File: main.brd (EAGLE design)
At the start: 130 x 34 mm, 176 parts, among them CN1 DC-012A-D010, CN2 JST GH 6P V-TH, CN3 5.8ZSPT, CN4 8 PIN FFC, CN5 MC-118LS-H100, CN6 JST GH 6P V-TH, CN7 8 PIN FFC, Q1 GSFP0449, Q6 IRLML6244, U1 Ti60F225C4, U10 W958D8NBYA5I, U11 TPS70918, U12 AP7335, U2 USBLC6-2SC6, U24 SCHMITT, U25 SCHMITT, U3 93LC56B-I/SN, U4 W25Q128JV, U5 TPS62065, U6 FT2232H, U7 TPS563201, U8 AR0822, U9 TPS62065

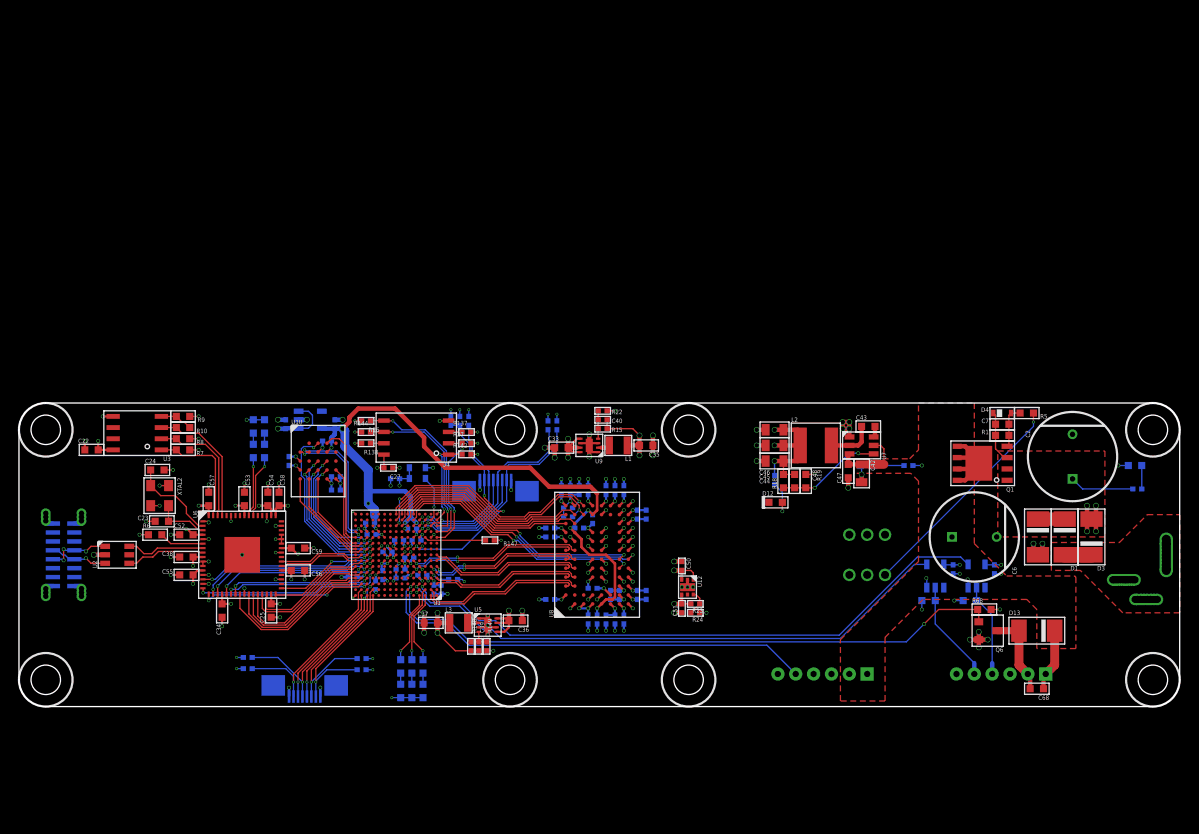
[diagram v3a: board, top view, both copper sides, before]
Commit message: Moving back to Trion
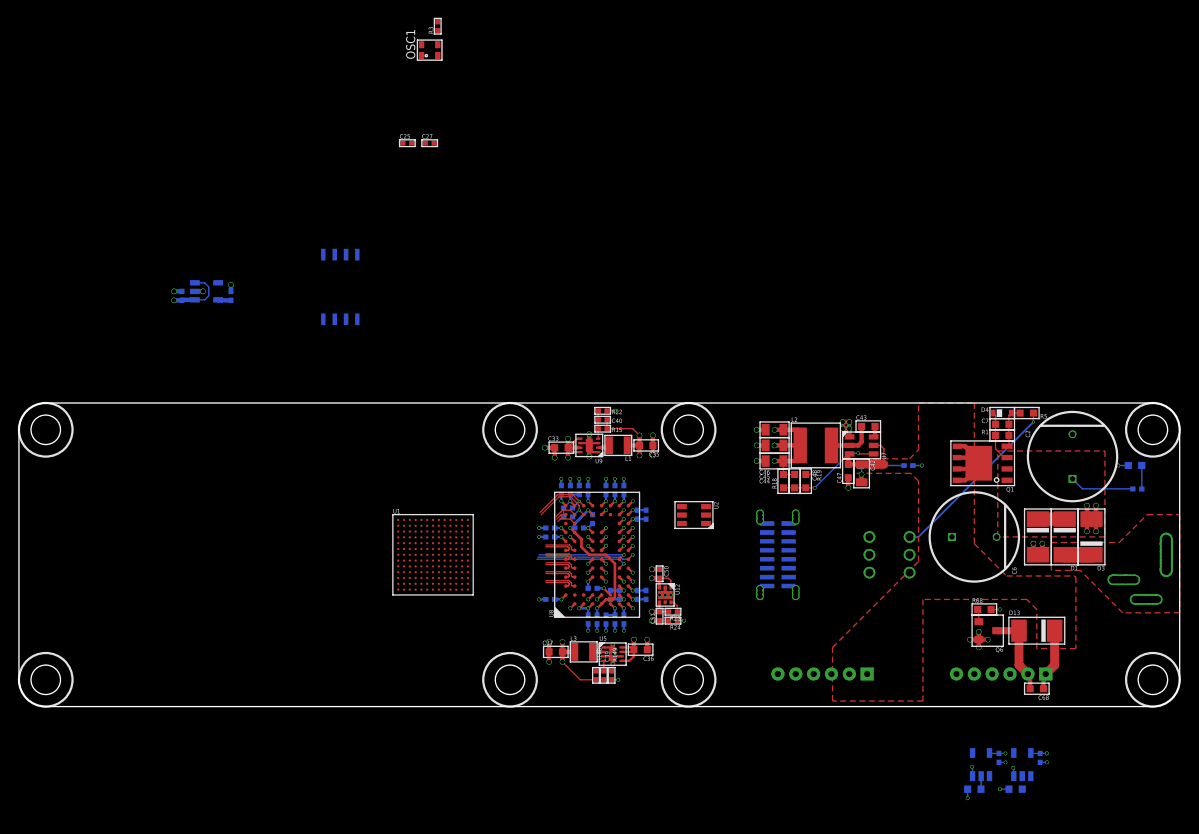
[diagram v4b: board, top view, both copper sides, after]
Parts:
- removed C22, C34, C38, C52, C53, C54, C55, C56, C57, C59: 0.1uF 16V, c_0603:0603
- removed C23, C24: 10pF 100V, c_0603:0603
- removed C28, C61, C62, C63, C64, C66, C67, C71, C72, C73, C74, C75, C77, C78, C79, C80, C81, C82: 0.1uF 16V, c_0402:0402
- removed C58: 4.7uF 6.3V, c_0603:0603
- removed C65, C76, C83: 10uF 6.3V, c_0402:0402
- removed CN4, CN7: 8 PIN FFC, CONNECTORs:SFV8R-1STBE1HLF
- removed D10, D12, D5, D6, D7, D8: RED LED, OPTO:0603_POLAR
- removed R10, R11, R12, R13, R14, R59: 2.2k, r_0603:0603
- removed R130, R137, R138, R142, R143, R144, R145, R146, R147, R20, R21, R26, R27, R74, R75: 10k, r_0402:0402
- removed R6: 12k, RESISTORS:0603
- removed R67: 1k, r_0402:0402
- removed R7, R8, R9: 10k, r_0603:0603
- removed U10: W958D8NBYA5I, ICs:VBGA24
- removed U3: 93LC56B-I/SN, ICs:SO8
- removed U4: W25Q128JV, ICs:SO8-208MIL
- removed U6: FT2232H, ICs:QFN64
- removed XTAL2: 12MHz, CRYSTALS:3.2X3.5SMD
- added U37: W25Q128JV, ICs:SO8-208MIL
- C25: value 0.1uF 16V -> 0.1uF 10V; device c_0603:0603 -> c_0402:0402
- C27: value 0.1uF 16V -> 0.1uF 10V
- R3: value 10k -> 10R
- U1: value Ti60F225C4 -> T20F169; device ICs:FBGA225 -> ICs:FBGA169
- moved CN5 80.0 mm to (20.0, 0.00), turned to 270 degrees
- moved U2 64.8 mm to (10.6, 4.45), turned to 270 degrees
- moved C25 54.5 mm to (-21.5, 46.1), turned to 0 degrees
- moved OSC1 47.4 mm to (-19.0, 56.5), flipped to the top, turned to 0 degrees
- moved R3 46.4 mm to (-18.1, 59.2), flipped to the top
- moved C27 36.6 mm to (-19.0, 46.1), turned to 0 degrees
- moved C69 21.7 mm to (49.4, -22.8)
- moved C70 21.7 mm to (44.8, -22.8)
- moved R72 21.7 mm to (46.6, -26.2)
- moved R73 21.7 mm to (42.0, -26.2)
- moved U24 21.7 mm to (47.4, -23.5)
- moved U25 21.7 mm to (42.8, -23.5)
- moved C41 18.5 mm to (-46.8, 29.0)
- moved C49 18.5 mm to (-41.2, 29.0)
- moved U11 18.5 mm to (-44.0, 29.5)
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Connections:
- removed net FLS_NHOLD: R138.1, U4.7
- removed net FLS_SPI_CLK: R144.1, U1.N1, U4.6
- removed net FLS_SPI_MISO: R27.1, U1.L1, U4.2
- removed net FLS_SPI_MOSI: R26.1, U1.M1, U4.5
- removed net FLS_SPI_NCS: R142.1, U1.P1, U4.1
- removed net FPGA_CLK_33M: OSC1.3, U1.P2
- removed net FPGA_CONF_CDONE: R147.1, U1.L3
- removed net FPGA_CONF_CSI: CN4.3, R145.1, U1.N2
- removed net FPGA_CONF_NCRST: C66.2, CN4.2, R146.1, U1.J5
- removed net FPGA_CONF_NTEST: R143.1, U1.E2
- removed net FPGA_JTAG_TCK: CN4.5, R3.1, U1.N4
- removed net FPGA_JTAG_TDI: CN4.4, U1.P3
- removed net FPGA_JTAG_TDO: CN4.7, R130.1, U1.M4
- removed net FPGA_JTAG_TMS: CN4.6, U1.N3
- removed net FT_CLKOUT: U1.G14, U6.32
- removed net FT_CONT_RX: U1.H14, U6.39
- removed net FT_CONT_TX: U1.G15, U6.38
- removed net FT_D0: U1.C13, U6.16
- removed net FT_D1: U1.C14, U6.17
- removed net FT_D2: U1.G13, U6.18
- removed net FT_D3: U1.F13, U6.19
- removed net FT_D4: U1.F12, U6.21
- removed net FT_D5: U1.E12, U6.22
- removed net FT_D6: U1.D13, U6.23
- removed net FT_D7: U1.C15, U6.24
- removed net FT_NOE: U1.H13, U6.33
- removed net FT_NRD: U1.E14, U6.28
- removed net FT_NRST: U1.H12, U6.14
- removed net FT_NRXF: U1.D14, U6.26
- removed net FT_NSIWU: U1.F15, U6.30
- removed net FT_NTXE: U1.D15, U6.27
- removed net FT_NWR: U1.E15, U6.29
- removed net LED_FPGA_STATUS: D6.K, U1.A4
- removed net LED_FT_CONT_NRXLED: D8.K, U6.54
- removed net LED_FT_CONT_NTXLED: D7.K, U6.55
- removed net LED_PROC_SCANNING: D10.K, U1.A3
- removed net LED_PROC_STATUS: D5.K, U1.B3
- removed net LED_USB_ACT: D12.K
- removed net N$113: D10.A, R59.1
- removed net N$14: D5.A, R11.1
- removed net N$15: D6.A, R12.1
- removed net N$16: D7.A, R13.1
- removed net N$17: D8.A, R14.1
- removed net N$42: R6.2, U6.6
- removed net N$43: R7.1, U3.1, U6.63
- removed net N$44: R8.1, U3.2, U6.62
- removed net N$45: R10.2, U3.3, U6.61
- removed net N$46: R10.1, R9.1, U3.4
- removed net N$47: D12.A, R67.1
- removed net N$49: C23.2, U6.3, XTAL2.3
- removed net N$50: C24.2, U6.2, XTAL2.1
- removed net N$51: C55.2, C56.2, C57.2, C58.2, U6.12, U6.37, U6.49, U6.64
- removed net N$8: R137.1, U4.3
- removed net PROC_JTAG_TCK: CN7.5, R21.1, U1.C12
- removed net PROC_JTAG_TDI: CN7.4, U1.A13
- removed net PROC_JTAG_TDO: CN7.7, R20.1, U1.B14
- removed net PROC_JTAG_TMS: CN7.6, U1.A14
- removed net PROC_UART_RX: CN7.2, R75.1, U1.A12
- removed net PROC_UART_TX: CN7.3, R74.1, U1.B12
- removed net PWR_MIPI_1V2: C75.2, C76.2, R143.2, U1.D2, U1.F4
- removed net RAM_CLKN: U1.M15, U10.B1
- removed net RAM_CLKP: U1.M14, U10.B2
- removed net RAM_D0: U1.K13, U10.D3
- removed net RAM_D1: U1.J13, U10.D2
- removed net RAM_D2: U1.L12, U10.C4
- removed net RAM_D3: U1.L13, U10.D4
- removed net RAM_D4: U1.K15, U10.D5
- removed net RAM_D5: U1.K14, U10.E3
- removed net RAM_D6: U1.J15, U10.E2
- removed net RAM_D7: U1.J14, U10.E1
- removed net RAM_NCS: U1.J12, U10.A3
- removed net RAM_NRESET: U1.L15, U10.A4
- removed net RAM_RWDS: U1.K12, U10.C3
- new net N$9: OSC1.3, R3.1
- new net PSS_CLK_33M: R3.2
- new net PSS_FLASH_D0: U37.5
- new net PSS_FLASH_D1: U37.2
- new net PSS_FLASH_D2: U37.3
- new net PSS_FLASH_D3: U37.7
- new net PSS_FLASH_NCS: U37.1
- new net PSS_FLASH_SCLK: U37.6
- new net USB_VBUS: CN5.A4, CN5.A9, CN5.B4, CN5.B9, U2.5
- net AR_CLK: no longer U1.P6
- net AR_GPIO0: no longer U1.P7
- net AR_GPIO1: no longer U1.R6
- net AR_GPIO2: no longer U1.P8
- net AR_GPIO3: no longer U1.R7
- net AR_I2C_SCL: no longer U1.R8
- net AR_I2C_SDA: no longer U1.N8
- net AR_MIPI_CLK_N: no longer U1.G1
- net AR_MIPI_CLK_P: no longer U1.H1
- net AR_MIPI_D0_N: no longer U1.F5
- net AR_MIPI_D0_P: no longer U1.G5
- net AR_MIPI_D1_N: no longer U1.F2
- net AR_MIPI_D1_P: no longer U1.F1
- net AR_MIPI_D2_N: no longer U1.C1
- net AR_MIPI_D2_P: no longer U1.D1
- net AR_MIPI_D3_N: no longer U1.A2
- net AR_MIPI_D3_P: no longer U1.B2
- net AR_NRESET: no longer U1.R5
- net AR_XSHUTDOWN: no longer U1.P5
- net GND: now also U37.4; no longer C22.1, C23.1, C24.1, C28.2, C34.1, C38.1, C52.1, C53.1, C54.1, C55.1, C56.1, C57.1, C58.1, C59.1, C61.1, C62.1, C63.1, C64.1, C65.1, C66.1, C67.1, C71.1, C72.1, C73.1, C74.1, C75.1, C76.1, C77.1, C78.1, C79.1, C80.1, C81.1, C82.1, C83.1, CN4.8, CN7.8, R6.1, U1.A1, U1.A15, U1.D3, U1.G6, U1.G8, U1.H7, U1.H9, U1.J6, U1.J8, U1.M13, U1.R1, U1.R15, U10.B3, U10.C1, U10.E5, U3.5, U4.4, U6.1, U6.10, U6.11, U6.13, U6.15, U6.25, U6.35, U6.41, U6.43, U6.44, U6.45, U6.47, U6.5, U6.51, U6.PAD, XTAL2.2, XTAL2.4
- net LED_PWM_CONT: no longer U1.C5
- net MTR_CONT_PWM: no longer U1.B5
- net MTR_SENSE_A: no longer U1.C3
- net MTR_SENSE_B: no longer U1.C4
- net PWR_FPGA_0V95: no longer C61.2, C62.2, C63.2, C64.2, C65.2, C67.2, C71.2, C72.2, C73.2, U1.E13, U1.E5, U1.G10, U1.G7, U1.G9, U1.H6, U1.H8, U1.J7, U1.J9, U1.L10, U1.L5, U1.M3
- net PWR_SYS_1V8: now also C25.2, OSC1.1, OSC1.4; no longer C74.2, C77.2, C78.2, C79.2, C80.2, C81.2, C82.2, C83.2, U1.D4, U1.E11, U1.J11, U1.L14, U1.L4, U1.M11, U1.N5, U1.N7, U10.B4, U10.D1, U10.E4
- net PWR_SYS_3V3: now also U37.8; no longer C22.2, C25.2, C28.1, C34.2, C38.2, C52.2, C53.2, C54.2, C59.2, CN4.1, CN7.1, OSC1.1, OSC1.4, R11.2, R12.2, R13.2, R130.2, R137.2, R138.2, R14.2, R142.2, R144.2, R145.2, R146.2, R147.2, R20.2, R21.2, R26.2, R27.2, R3.2, R59.2, R67.2, R7.2, R74.2, R75.2, R8.2, R9.2, U1.B13, U1.B4, U1.F14, U1.G12, U1.J4, U1.L2, U1.P4, U3.8, U4.8, U6.20, U6.31, U6.4, U6.42, U6.50, U6.56, U6.59, U6.9
- net USB_D_N: no longer U6.7
- net USB_D_P: no longer U6.8
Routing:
- net PWR_SYS_1V8: track 126.2 -> 27.1 mm, vias 17 -> 4
- net MTR_CONT_PWM: track 70.6 -> 1.43 mm, vias 2 -> 0
- net MTR_SENSE_A: track 68.3 -> 0.00 mm, vias 1 -> 0
- net MTR_SENSE_B: track 63.9 -> 0.00 mm, vias 1 -> 0
- net GND: track 161.7 -> 100.7 mm, vias 156 -> 97
- net PWR_SYS_3V3: track 95.1 -> 43.9 mm, vias 50 -> 10
- net LED_PWM_CONT: track 50.0 -> 0.00 mm, vias 1 -> 0
- net N$51: track 36.7 -> 0.00 mm, vias 4 -> 0
- net FPGA_CONF_NCRST: track 25.1 -> 0.00 mm, vias 3 -> 0
- net FPGA_JTAG_TDO: track 23.9 -> 0.00 mm, vias 1 -> 0
- net FPGA_JTAG_TCK: track 23.0 -> 0.00 mm, vias 1 -> 0
- net PROC_JTAG_TCK: track 22.7 -> 0.00 mm, vias 3 -> 0
- net AR_GPIO2: track 24.1 -> 2.64 mm
- net AR_I2C_SDA: track 28.5 -> 7.28 mm, vias 3 -> 1
- net PROC_UART_TX: track 21.0 -> 0.00 mm, vias 1 -> 0
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- added copper zone on layer 3, net PWR_DDR3_1V35
- removed copper zone on layer 3, net PWR_FPGA_0V95
